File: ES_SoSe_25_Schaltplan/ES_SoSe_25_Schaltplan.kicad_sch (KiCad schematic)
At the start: 8 parts

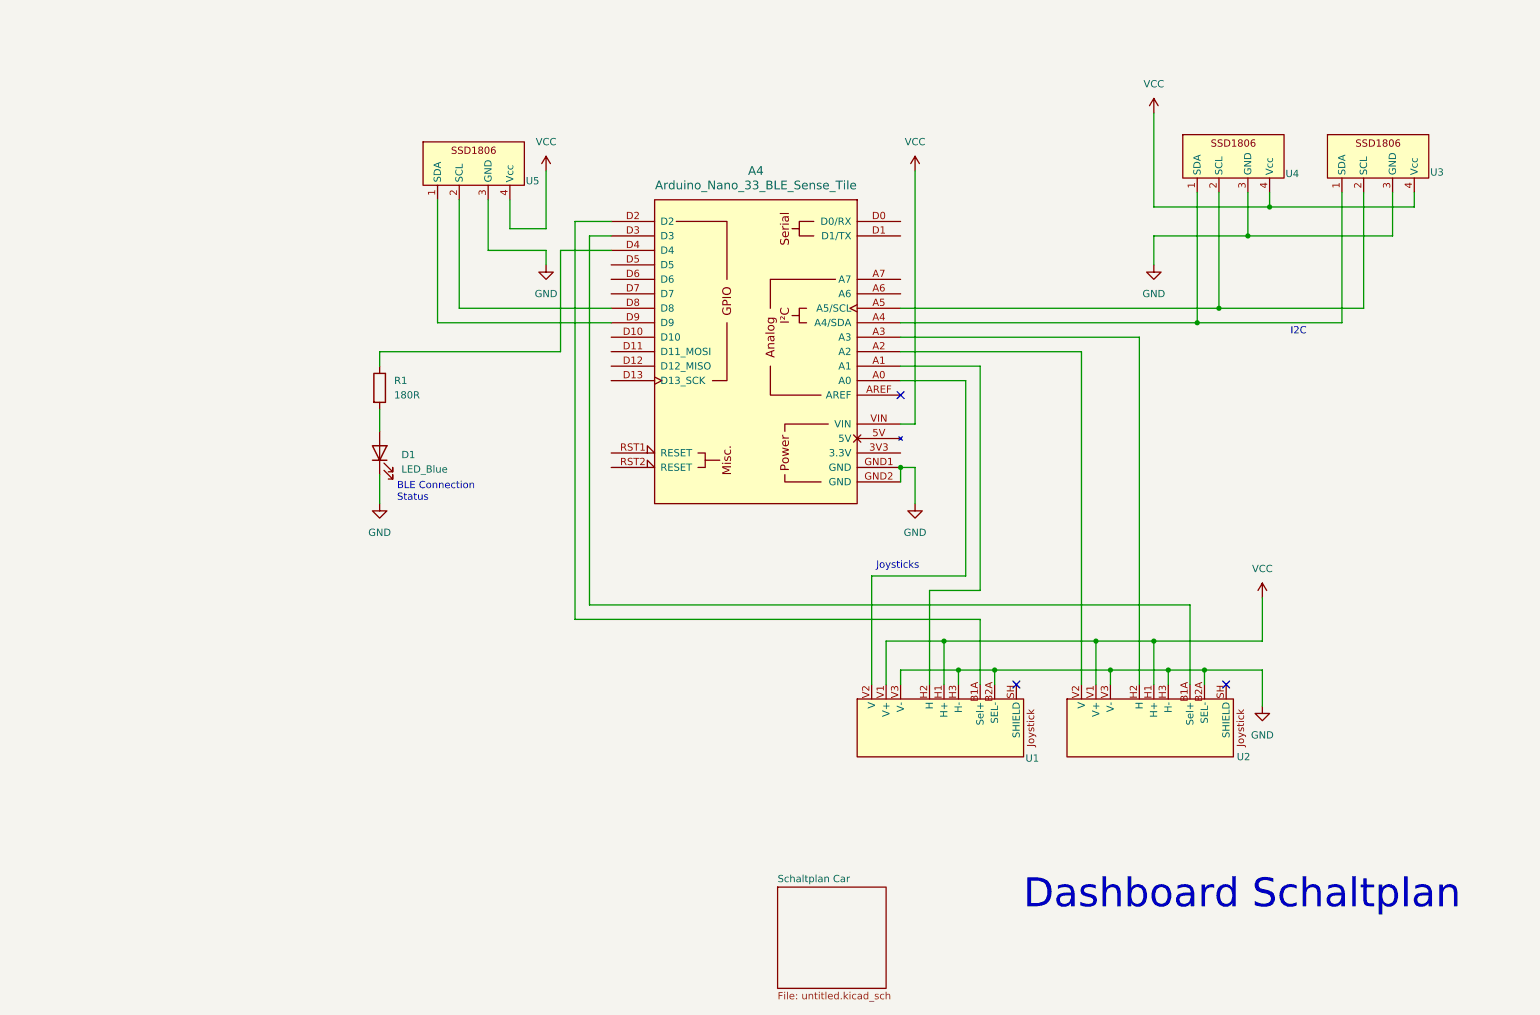
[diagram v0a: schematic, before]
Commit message: edited ble and scematic
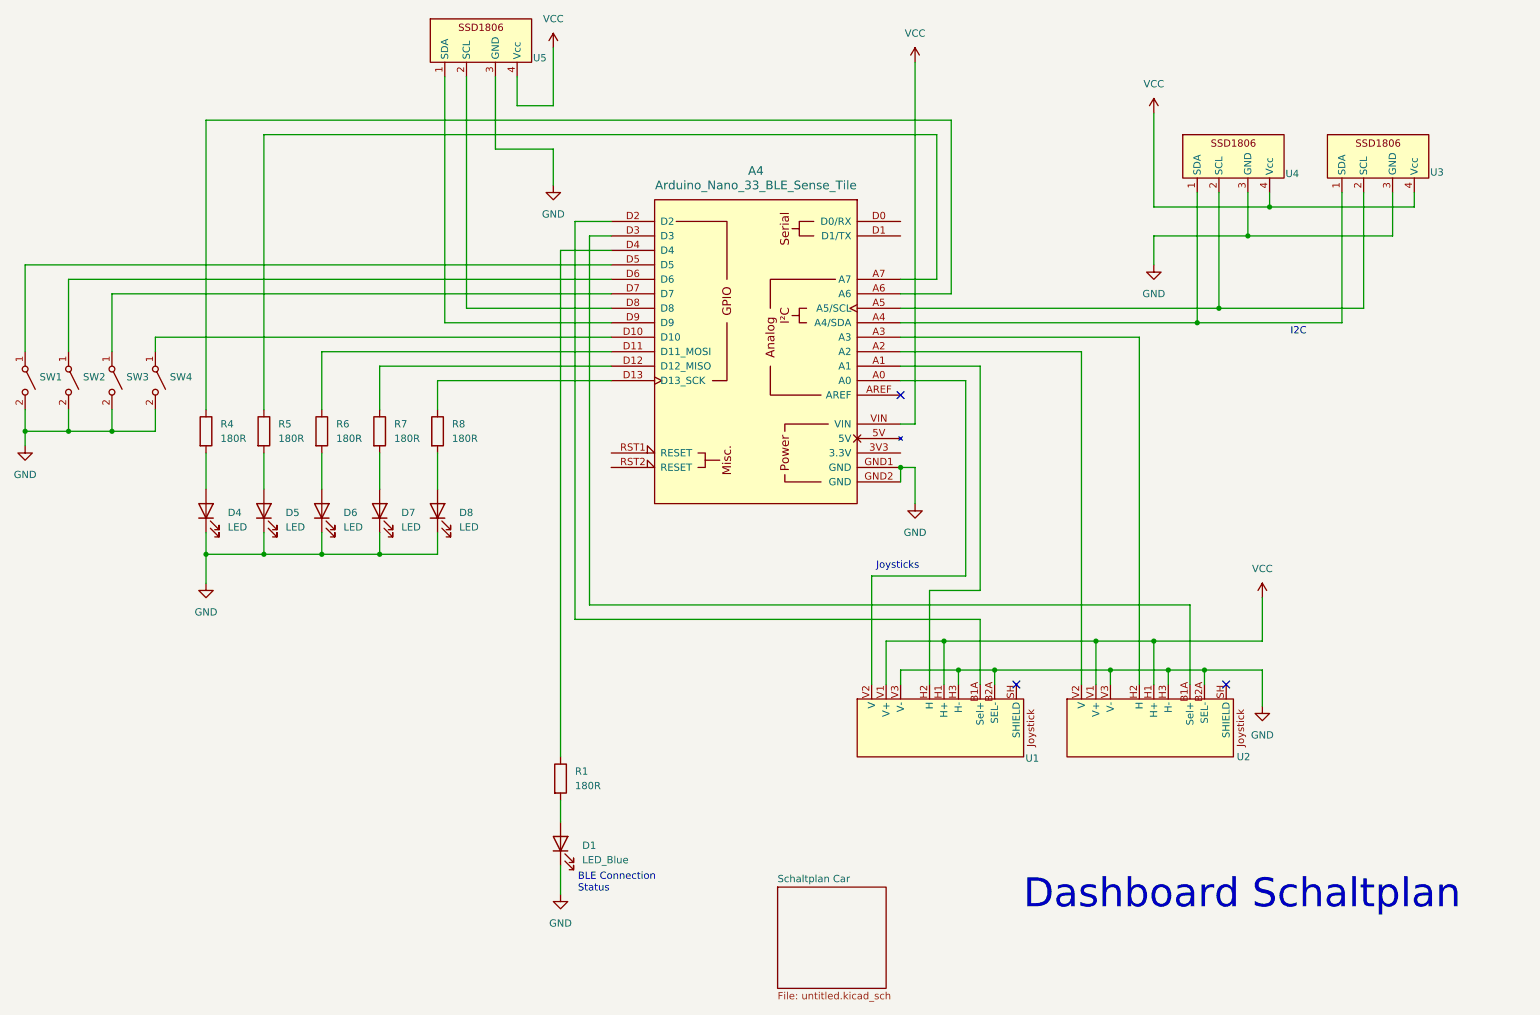
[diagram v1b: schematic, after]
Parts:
- added D4, D5, D6, D7, D8: LED, symbol Device:LED
- added R4, R5, R6, R7, R8: 180R, symbol Device:R
- added SW1, SW2, SW3, SW4: ~, symbol Switch:SW_SPST
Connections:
- net GND: now also D4.1 (K), D5.1 (K), D6.1 (K), D7.1 (K), D8.1 (K), SW1.2 (B), SW2.2 (B), SW3.2 (B), SW4.2 (B)
- net at A4.A6: now also R4.1
- net at A4.A7: now also R5.1
- net at A4.D10: now also SW4.1 (A)
- net at A4.D11 (D11_MOSI): now also R6.1
- net at A4.D12 (D12_MISO): now also R7.1
- net at A4.D13 (D13_SCK): now also R8.1
- net at A4.D5: now also SW1.1 (A)
- net at A4.D6: now also SW2.1 (A)
- net at A4.D7: now also SW3.1 (A)
- new net: D5.2 (A), R5.2
- new net: D6.2 (A), R6.2
- new net: D4.2 (A), R4.2
- new net: D8.2 (A), R8.2
- new net: D7.2 (A), R7.2
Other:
- moved on the sheet: D1, R1, U5
